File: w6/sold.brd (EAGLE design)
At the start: 101.5 x 80.5 mm, 35 parts, among them T1 50v 16A N-channel, U1 AD8615AUJ, U2 AD8615AUJ

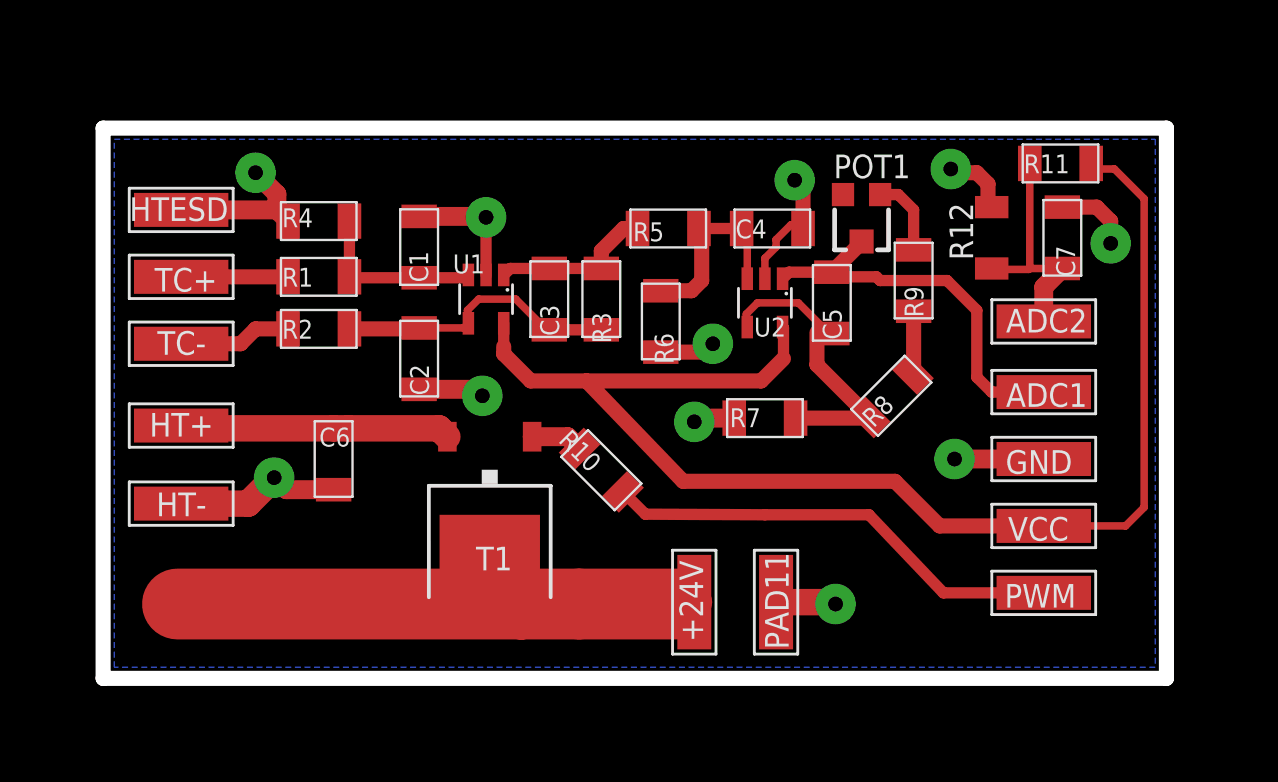
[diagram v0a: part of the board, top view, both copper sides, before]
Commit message: shopbot done and many other typos and w6 8 9 10 11 12 proof
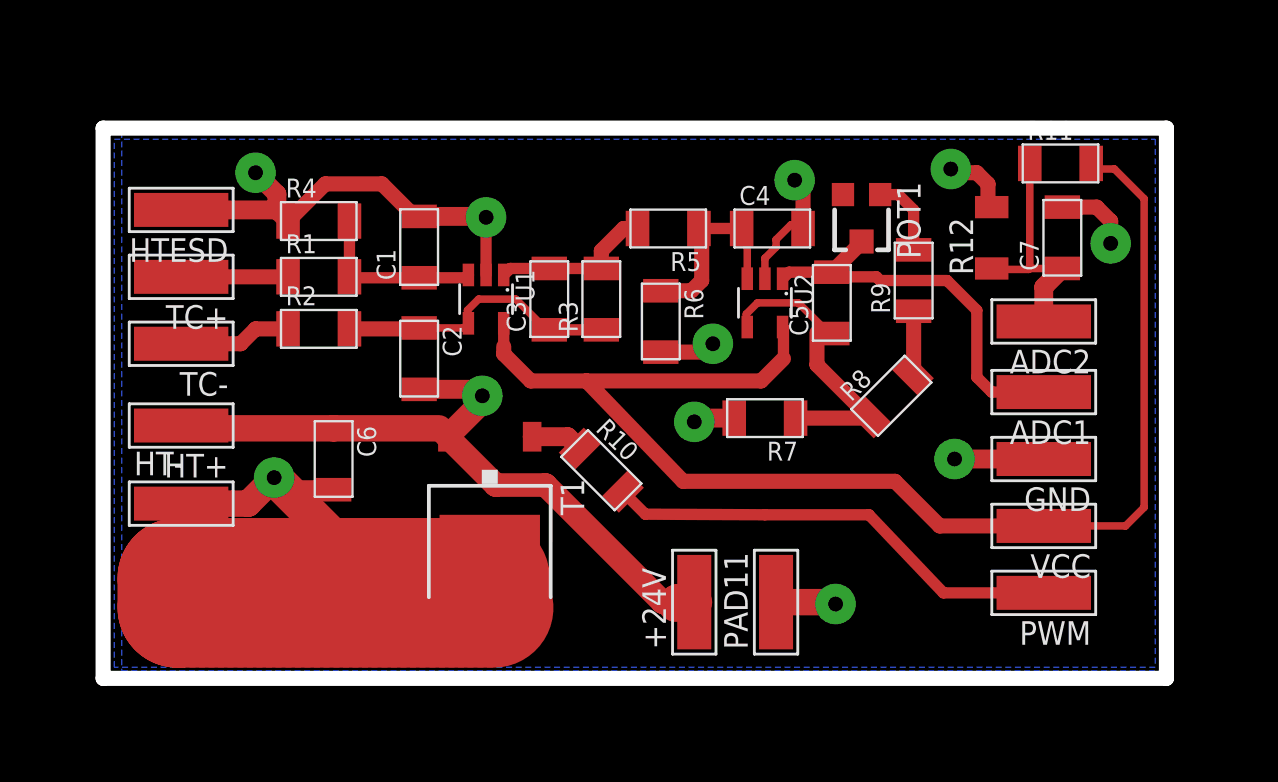
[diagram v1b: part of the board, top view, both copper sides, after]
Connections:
- removed net N$9: C6.1, HT+.1, T1.2
- new net N$15: C6.2, HT-.1, T1.3
- net GND: now also T1.2; no longer C6.2, HT-.1
- net N$14: now also C6.1, HT+.1; no longer T1.3
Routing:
- net N$15: track 0.00 -> 22.8 mm, vias 0 -> 1
- net N$9: track 14.6 -> 35.4 mm
- net GND: track 56.7 -> 59.1 mm, vias 11 -> 10
- net N$14: track 30.2 -> 32.0 mm
